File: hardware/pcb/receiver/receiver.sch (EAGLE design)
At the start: 79 parts, among them X1 5-1634506-1H

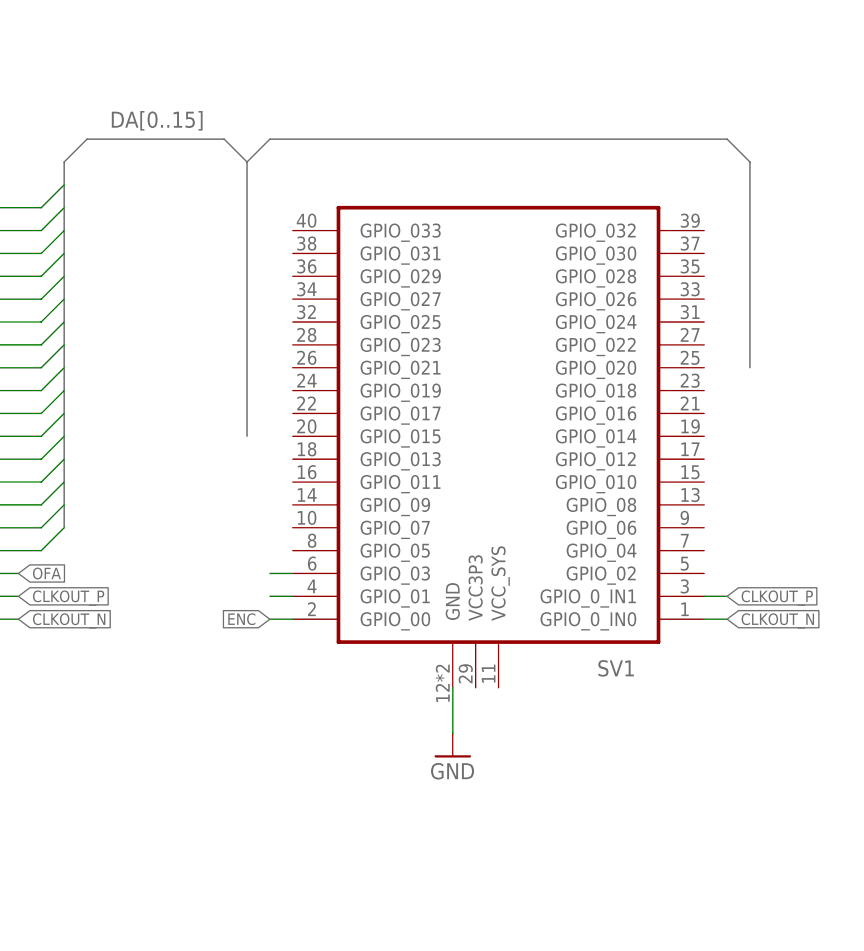
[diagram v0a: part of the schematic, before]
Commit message: hw: board updates
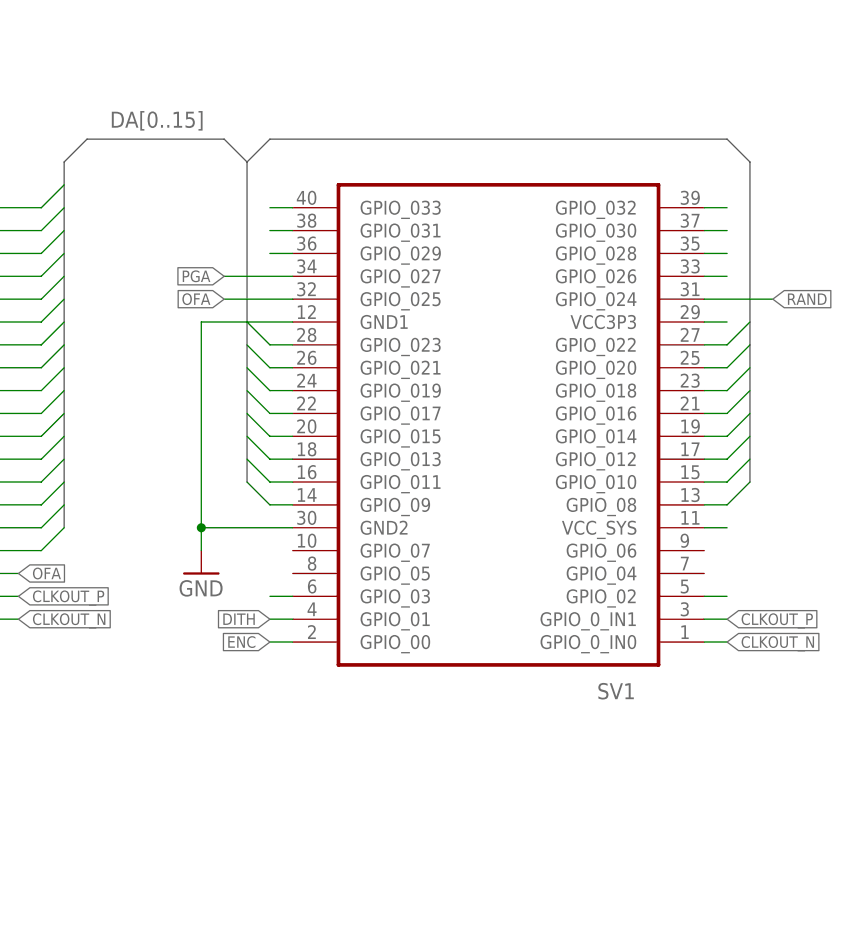
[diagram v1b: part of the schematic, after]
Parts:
- SV1: MFR 929975-01-20 -> (none)
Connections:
- removed net N$34: SV1.GPIO_01
- new net N$32: SV1.GPIO_029
- new net N$35: SV1.GPIO_031
- new net N$36: SV1.GPIO_033
- new net N$37: SV1.GPIO_032
- new net N$38: SV1.GPIO_030
- new net N$45: SV1.GPIO_028
- new net N$46: SV1.GPIO_026
- new net N$48: SV1.VCC3P3
- new net N$52: SV1.GPIO_02
- new net N$58: SV1.VCC_SYS
- net DA0: now also SV1.GPIO_08
- net DA1: now also SV1.GPIO_09
- net DA10: now also SV1.GPIO_018
- net DA11: now also SV1.GPIO_019
- net DA12: now also SV1.GPIO_020
- net DA13: now also SV1.GPIO_021
- net DA14: now also SV1.GPIO_022
- net DA15: now also SV1.GPIO_023
- net DA2: now also SV1.GPIO_010
- net DA3: now also SV1.GPIO_011
- net DA4: now also SV1.GPIO_012
- net DA5: now also SV1.GPIO_013
- net DA6: now also SV1.GPIO_014
- net DA7: now also SV1.GPIO_015
- net DA8: now also SV1.GPIO_016
- net DA9: now also SV1.GPIO_017
- net DITH: now also SV1.GPIO_01
- net GND: now also SV1.GND1, SV1.GND2; no longer SV1.GND
- net OFA: now also SV1.GPIO_025
- net PGA: now also SV1.GPIO_027
- net RAND: now also SV1.GPIO_024
